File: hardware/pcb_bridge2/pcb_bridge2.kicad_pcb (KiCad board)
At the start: 2 copper layers, 12.3 x 17.9 mm, 2 parts, among them J1 68710614522, J2 687108149022

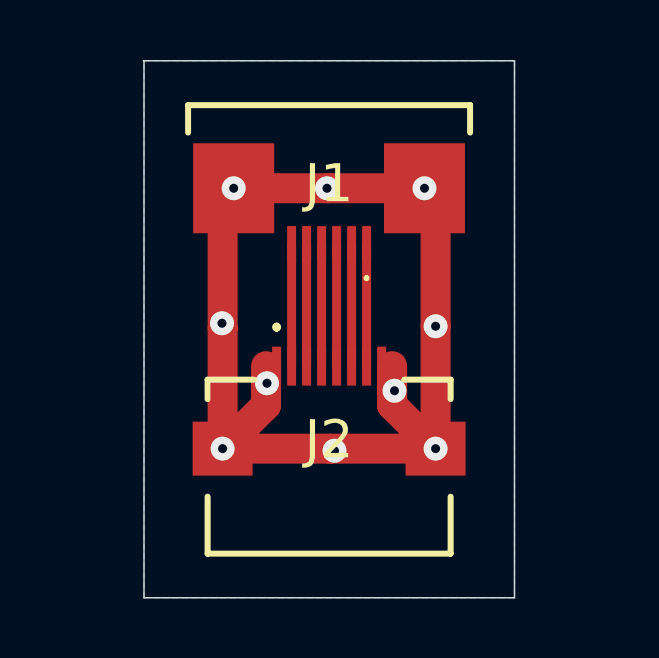
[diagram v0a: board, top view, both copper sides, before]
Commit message: both bridge finished
main pcb layout nearly there
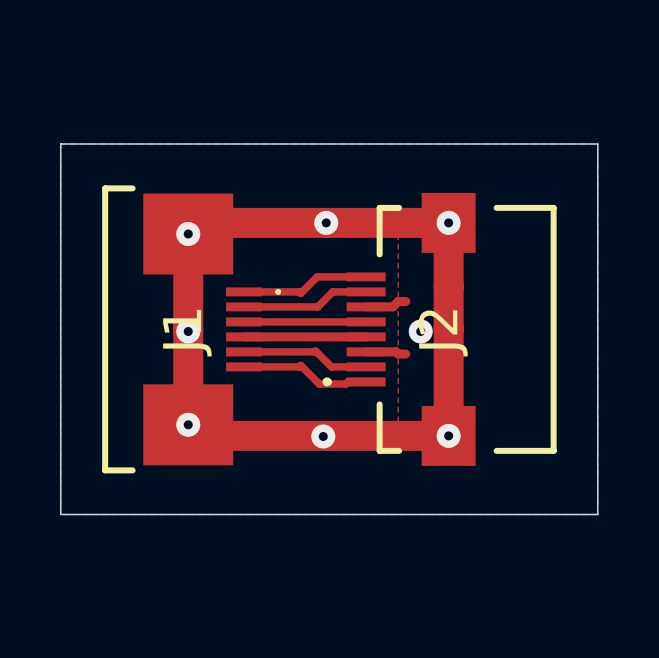
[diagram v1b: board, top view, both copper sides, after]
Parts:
- moved J1 6.87 mm to (116.0, 52.2), turned to -90 degrees
- moved J2 5.63 mm to (124.8, 52.2), turned to 90 degrees
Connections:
- J2 pad 1: AVSS -> Net-(J1-Pad6)
- J2 pad 2: Net-(J1-Pad6) -> Net-(J1-Pad5)
- J2 pad 3: Net-(J1-Pad5) -> AVSS
- J2 pad 6: Net-(J1-Pad2) -> AVSS
- J2 pad 7: Net-(J1-Pad1) -> Net-(J1-Pad2)
- J2 pad 8: AVSS -> Net-(J1-Pad1)
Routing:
- net AVSS: track 38.5 -> 34.6 mm, vias 10 -> 8
- added copper zone on F.Cu, net AVSS
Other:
- board size 12.3 x 17.9 mm -> 17.9 x 12.4 mm
